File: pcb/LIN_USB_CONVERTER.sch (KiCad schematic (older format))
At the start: 33 parts, among them J1 Conn_01x03, J2 TerminalBlock, J3 GS2, J4 USB_A, J5 Conn_01x02, P2 CONN_01X05, U1 TJA1028TK/3V3/20/J, U2 MAX12931BASA+, U3 MCP1700T-3302E/TT, U4 STM32F042G4U6

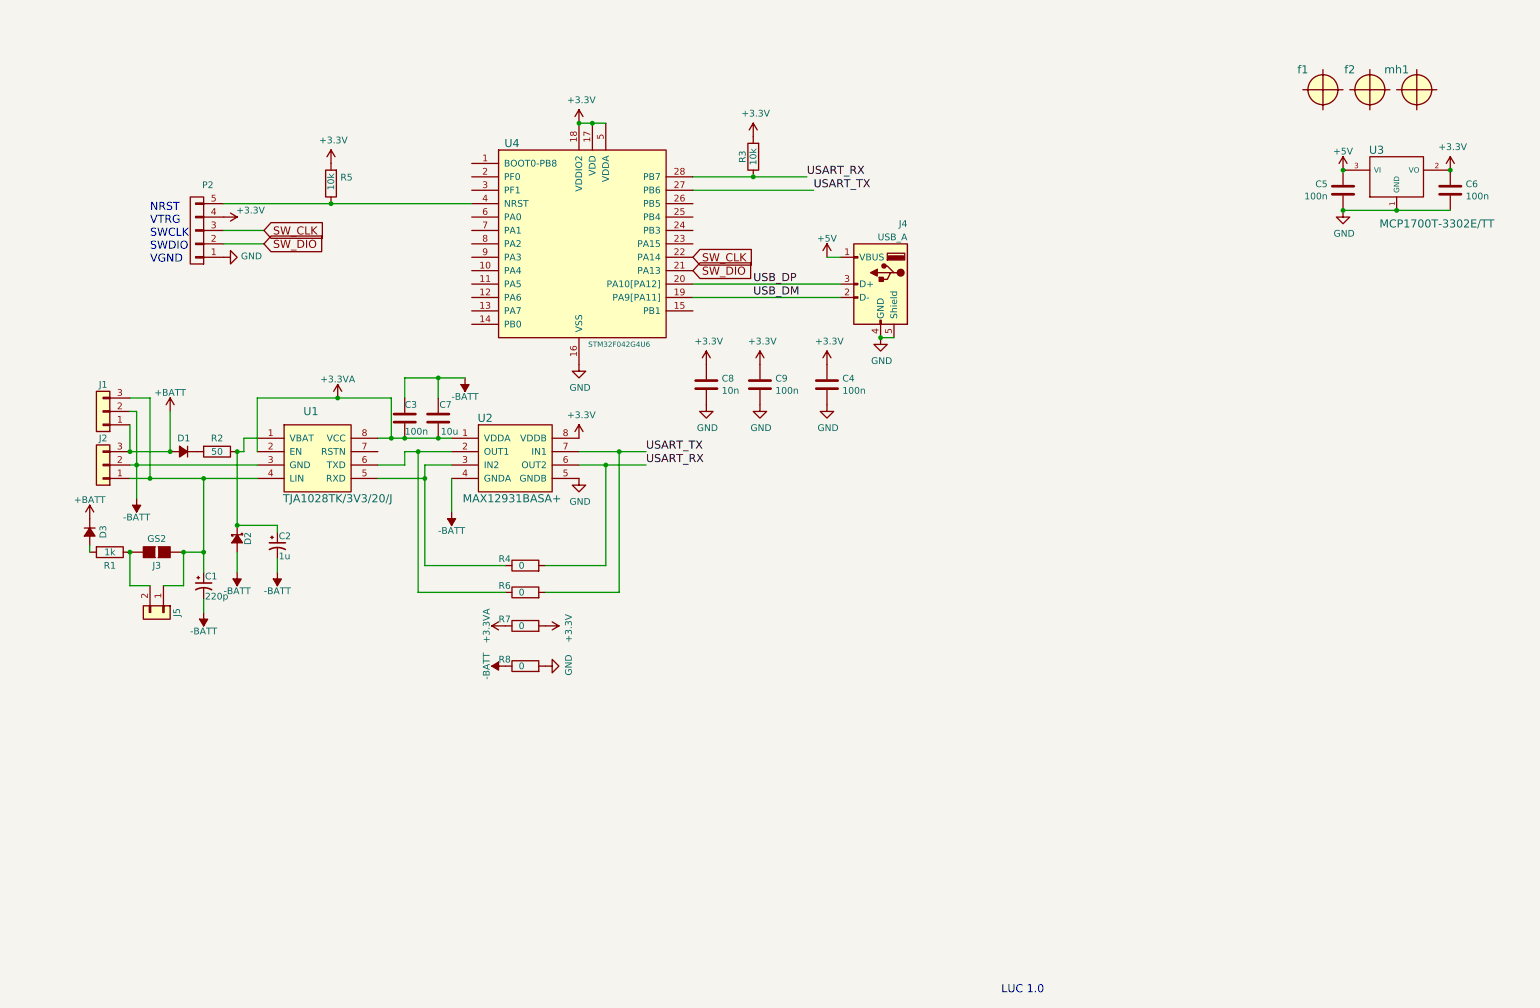
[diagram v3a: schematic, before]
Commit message: PCB release
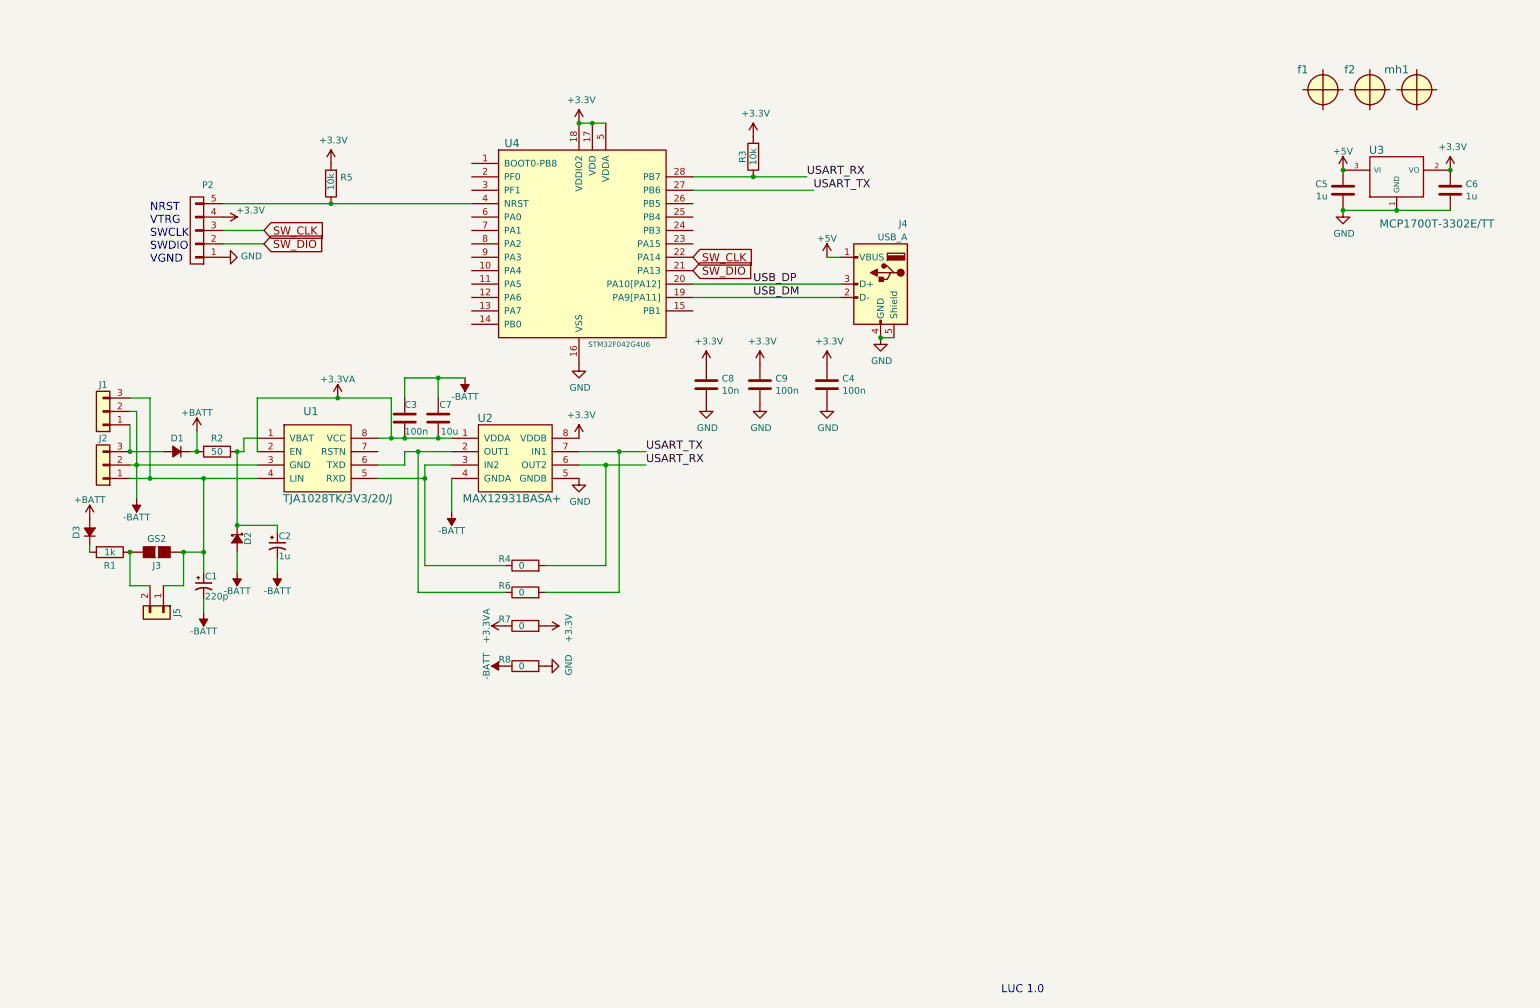
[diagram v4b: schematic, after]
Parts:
- C5, C6: value 100n -> 1u
- C7: footprint Capacitors_SMD:C_0402 -> Capacitors_SMD:C_0603
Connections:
- net +BATT: now also D1.1 (K), D3.2 (A), R2.2; no longer D1.2 (A), D3.1 (K), J1.1 (Pin_1), J2.3 (Pin_3)
- net at R1.2: now also D3.1 (K); no longer D3.2 (A)
- new net: D1.2 (A), J1.1 (Pin_1), J2.3 (Pin_3)
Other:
- moved on the sheet: D1
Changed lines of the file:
@@
 L LIN_USB_CONVERTER-rescue:+BATT-RESCUE-LIN_USB_CONVERTER #PWR010
 U 1 1 5A6A2468
-P 1200 3150
-F 0 "#PWR010" H 1200 3000 50  0001 C CNN
-F 1 "+BATT" H 1200 3290 50  0000 C CNN
-F 2 "" H 1200 3150 50  0001 C CNN
-F 3 "" H 1200 3150 50  0001 C CNN
-	1    1200 3150
+P 1400 3300
+F 0 "#PWR010" H 1400 3150 50  0001 C CNN
+F 1 "+BATT" H 1400 3440 50  0000 C CNN
+F 2 "" H 1400 3300 50  0001 C CNN
+F 3 "" H 1400 3300 50  0001 C CNN
+	1    1400 3300
 	1    0    0    -1
 $EndComp
@@
 L LIN_USB_CONVERTER-rescue:D_Small_ALT-RESCUE-LIN_USB_CONVERTER D1
 U 1 1 5A6A2C4B
-P 1300 3450
-F 0 "D1" H 1250 3350 50  0000 L CNN
-F 1 "SMBD914E6327HTSA1" H 1150 3370 50  0001 L CNN
-F 2 "Diodes_SMD:D_SOT-23_ANK" V 1300 3450 50  0001 C CNN
-F 3 "" V 1300 3450 50  0001 C CNN
-F 4 "https://www.tme.eu/pl/details/smbd914e6327htsa1/diody-uniwersalne-smd/infineon-technologies/" H 1300 3450 50  0001 C CNN "1st Disrtib Link"
-F 5 "INFINEON " H 1300 3450 50  0001 C CNN "Manufacturer"
-	1    1300 3450
+P 1250 3450
+F 0 "D1" H 1200 3350 50  0000 L CNN
+F 1 "SMBD914E6327HTSA1" H 1100 3370 50  0001 L CNN
+F 2 "Diodes_SMD:D_SOT-23_ANK" V 1250 3450 50  0001 C CNN
+F 3 "" V 1250 3450 50  0001 C CNN
+F 4 "https://www.tme.eu/pl/details/smbd914e6327htsa1/diody-uniwersalne-smd/infineon-technologies/" H 1250 3450 50  0001 C CNN "1st Disrtib Link"
+F 5 "INFINEON " H 1250 3450 50  0001 C CNN "Manufacturer"
+	1    1250 3450
 	-1   0    0    1
 $EndComp
@@
 P 9950 1500
 F 0 "C5" H 10065 1546 50  0000 L CNN
-F 1 "100n" H 10065 1455 50  0000 L CNN
+F 1 "1u" H 10065 1455 50  0000 L CNN
 F 2 "Capacitors_SMD:C_0402" H 9988 1350 50  0001 C CNN
 F 3 "" H 9950 1500 50  0000 C CNN
@@
 P 10750 1500
 F 0 "C6" H 10865 1546 50  0000 L CNN
-F 1 "100n" H 10865 1455 50  0000 L CNN
+F 1 "1u" H 10865 1455 50  0000 L CNN
 F 2 "Capacitors_SMD:C_0402" H 10788 1350 50  0001 C CNN
 F 3 "" H 10750 1500 50  0000 C CNN
@@
 F 0 "C7" H 3100 3300 50  0000 L CNN
 F 1 "10u" H 3050 3100 50  0000 L CNN
-F 2 "Capacitors_SMD:C_0402" H 3238 3050 50  0001 C CNN
+F 2 "Capacitors_SMD:C_0603" H 3238 3050 50  0001 C CNN
 F 3 "" H 3200 3200 50  0000 C CNN
 F 4 "https://www.tme.eu/pl/details/cl05a106mq5nunc/kondensatory-mlcc-smd-0402/samsung/" H 3200 3200 50  0001 C CNN "1st Disrtib Link"
@@
 	3100 3650 2750 3650
 Wire Wire Line
-	1200 3450 1200 3150
-Connection ~ 1200 3450
-Wire Wire Line
 	1700 3450 1750 3450
-Wire Wire Line
-	900  3450 1200 3450
 Wire Wire Line
 	1700 4000 2000 4000
@@
 Wire Wire Line
 	900  3450 900  3250
-Connection ~ 900  3450
 Connection ~ 3200 3350
 Wire Wire Line
@@
 F 5 "INFINEON " H 600 4050 50  0001 C CNN "Manufacturer"
 	1    600  4050
-	0    1    1    0
+	0    -1   -1   0
 $EndComp
 Wire Wire Line
@@
 Wire Wire Line
 	2950 3350 3200 3350
+Wire Wire Line
+	1400 3300 1400 3450
+Wire Wire Line
+	1400 3450 1350 3450
+Connection ~ 1400 3450
+Wire Wire Line
+	1150 3450 900  3450
+Connection ~ 900  3450
 $EndSCHEMATC
